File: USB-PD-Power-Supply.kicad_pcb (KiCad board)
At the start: 2 copper layers, 40 parts, among them IC1 MC14051BDR2G, J1 Screw_Terminal_01x02, J2 USB_C_Receptacle_USB2.0_16P, J3 Conn_01x03_Pin, Q1 2N7002, U1 SW-SMD_DSHP03TS-S, U2 CH224A, U3 TPS70933DBVR

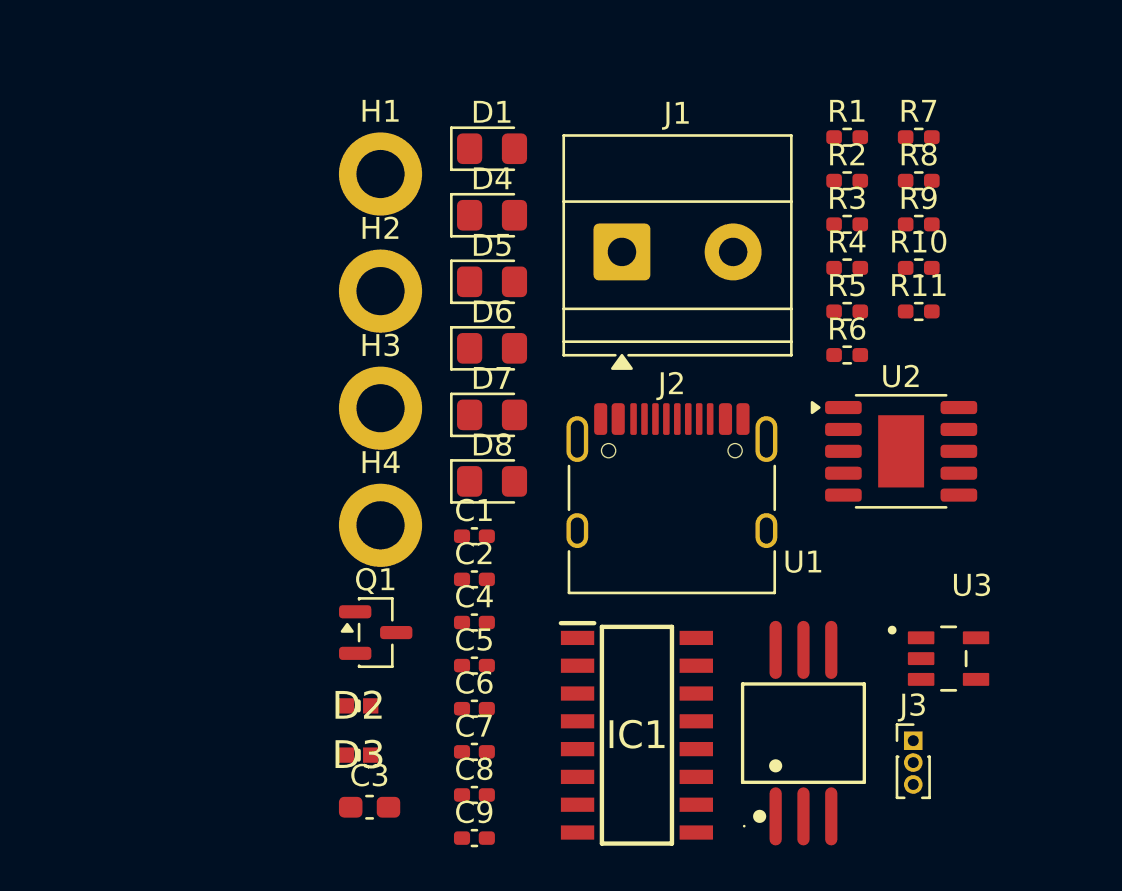
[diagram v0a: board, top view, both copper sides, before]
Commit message: Completed Routing, Adjusted Silkscreen, and Images
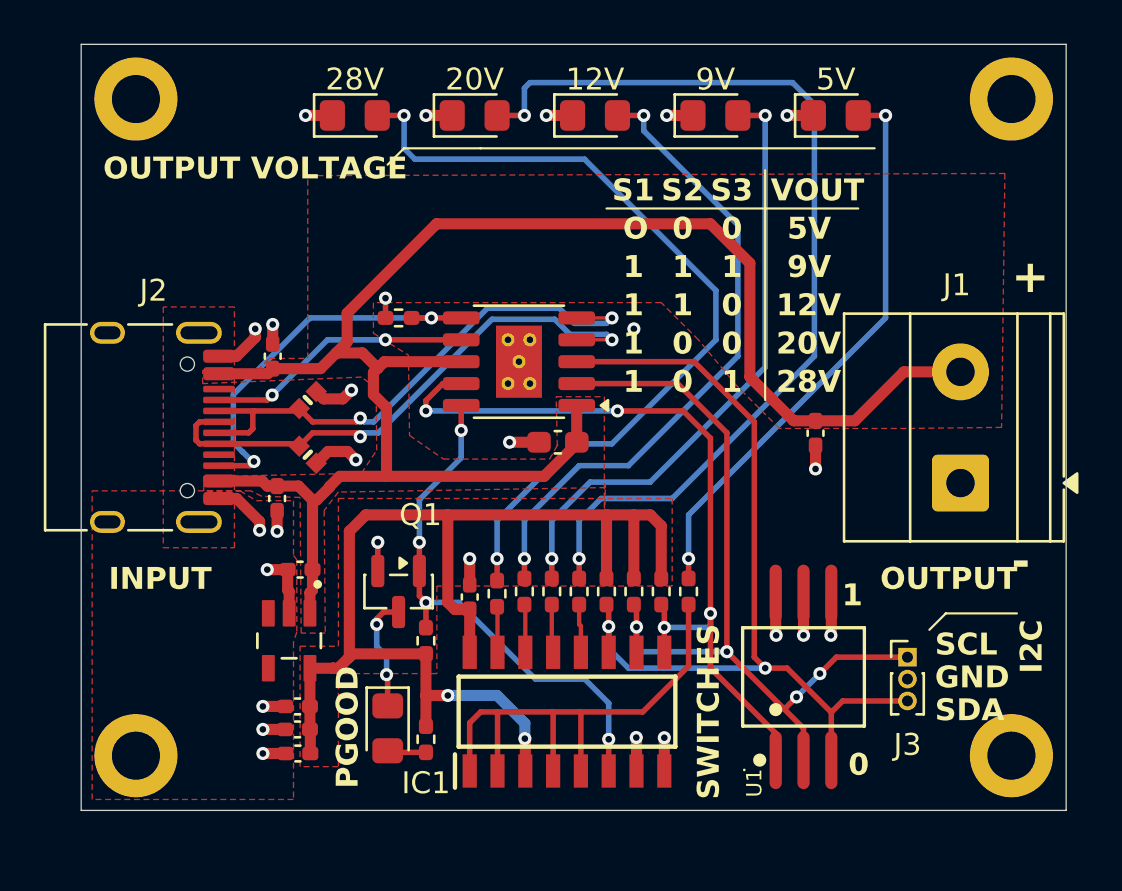
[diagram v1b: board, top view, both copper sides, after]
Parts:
- moved R1 33.6 mm to (141.0, 117.8), turned to -90 degrees
- moved H4 30.7 mm to (167.8, 118.5)
- moved U3 30.1 mm to (134.8, 113.2), turned to -90 degrees
- moved H2 30.1 mm to (167.8, 88.5)
- moved R2 28.5 mm to (141.0, 113.2), turned to 90 degrees
- moved R7 28.4 mm to (144.2, 111.1), turned to -90 degrees
- moved D1 26.9 mm to (139.2, 117.2), turned to -90 degrees
- moved J2 25.0 mm to (127.5, 103.5), turned to -90 degrees
- moved R9 24.6 mm to (145.5, 111.0), turned to -90 degrees
- moved R8 24.3 mm to (148.0, 111.0), turned to -90 degrees
- moved 5V 22.9 mm to (159.7, 89.2)
- moved R10 22.4 mm to (146.8, 111.0), turned to -90 degrees
- moved R6 20.6 mm to (139.8, 98.5), turned to 180 degrees
- moved H3 19.4 mm to (127.8, 118.5)
- moved R3 18.8 mm to (151.8, 111.0), turned to -90 degrees
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- renumbered D6 to 12V, D5 to 20V, D4 to 28V, D8 to 5V, D7 to 9V
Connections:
- D2 pad 1: /USB_P -> /USB_N
- D3 pad 1: /USB_N -> /USB_P
- IC1 pad 11: /CFB1 -> /CFB3_SDA
- IC1 pad 9: /CFB3_SDA -> /CFB1
- J1 pad 1: V_USB -> GND
- J1 pad 2: GND -> V_USB
- J2 pad A6: /USB_N -> /USB_P
- J2 pad A7: /USB_P -> /USB_N
- J2 pad B6: /USB_N -> /USB_P
- J2 pad B7: /USB_P -> /USB_N
- U2 pad 4: /USB_N -> /USB_P
- U2 pad 5: /USB_P -> /USB_N
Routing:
- net V_USB: track 0.00 -> 81.3 mm
- net +3.3V: track 0.00 -> 55.8 mm, vias 0 -> 2
- net Net-(D5-A): track 0.00 -> 44.5 mm, vias 0 -> 2
- net /CFB3_SDA: track 0.00 -> 41.2 mm, vias 0 -> 2
- net /CFB2_SCL: track 0.00 -> 38.4 mm, vias 0 -> 4
- net Net-(D4-A): track 0.00 -> 38.2 mm, vias 0 -> 2
- net GND: track 0.00 -> 37.8 mm, vias 0 -> 26
- net /CFB1: track 0.00 -> 36.8 mm, vias 0 -> 4
- net Net-(D6-A): track 0.00 -> 29.7 mm, vias 0 -> 2
- net Net-(D7-A): track 0.00 -> 28.3 mm, vias 0 -> 2
- net Net-(D8-A): track 0.00 -> 26.1 mm, vias 0 -> 2
- net /USB_P: track 0.00 -> 25.3 mm, vias 0 -> 2
- net /USB_N: track 0.00 -> 24.9 mm, vias 0 -> 2
- net /PG: track 0.00 -> 24.4 mm, vias 0 -> 4
- net Net-(IC1-X4): track 0.00 -> 24.0 mm
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- added copper zone on F.Cu, net +3.3V
- added copper zone on F.Cu, net GND
- added copper zone on In1.Cu, net GND
- added copper zone on In2.Cu, net GND
- added copper zone on F.Cu, net V_USB
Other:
- board outline added: 45 x 35 mm
- copper layers 2 -> 4
- board text added: "+"
- board text added: "-"
- board text added: "0"
- board text added: "1"
- board text added: "12V"
- board text added: "20V"
- board text added: "28V"
- board text added: "5V"
- board text added: "9V"
- board text added: "GND"
- board text added: "I2C"
- board text added: "INPUT"
- board text added: "O"
- board text added: "OUTPUT"
- board text added: "OUTPUT VOLTAGE"
- board text added: "PGOOD"
- board text added: "S1"
- board text added: "S2"
- board text added: "S3"
- board text added: "SCL"
- board text added: "SDA"
- board text added: "SWITCHES"
- board text added: "VOUT"
